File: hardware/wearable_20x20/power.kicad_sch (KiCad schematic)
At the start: 27 parts, among them U1 BQ25185, U2 TPS7A2033PDBVR, U3 TPS63802DLAR, U4 TPS22917DBVR, U5 TPS22917DBVR

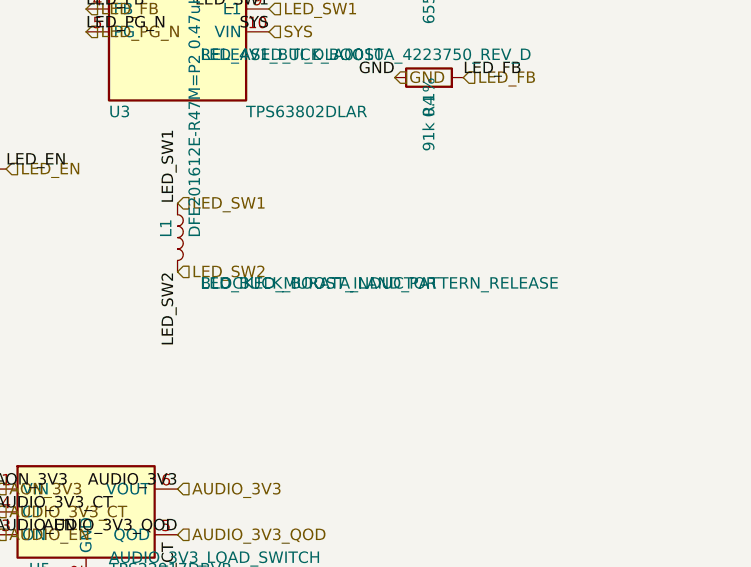
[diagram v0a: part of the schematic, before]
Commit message: Release crystal and power inductor packages
Co-authored-by: illiapliukhin <illiapliukhin@users.noreply.github.com>
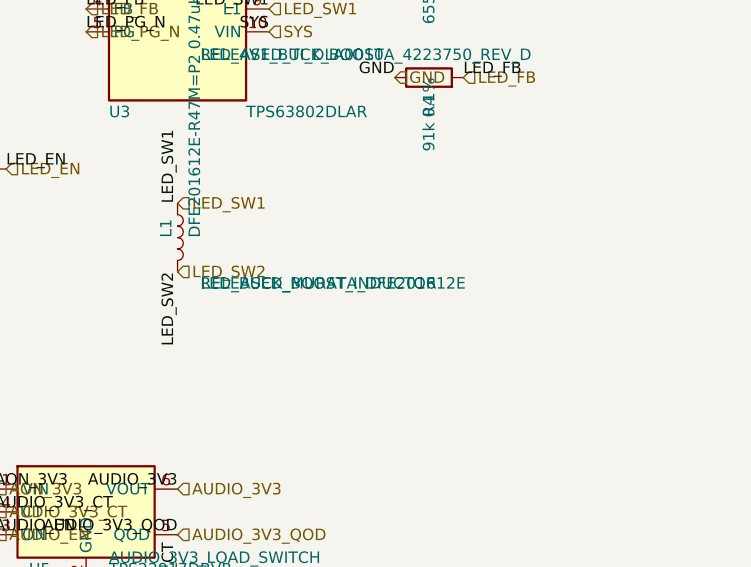
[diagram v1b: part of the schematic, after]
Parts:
- L1: footprint (none) -> PartSignal_Packages:Murata_DFE201612E_2.0x1.6mm; FootprintStatus BLOCKED_MURATA_LAND_PATTERN_RELEASE -> RELEASED_MURATA_DFE201612E
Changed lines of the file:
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@@
 			)
 		)
-		(property "Footprint" ""
+		(property "Footprint" "PartSignal_Packages:Murata_DFE201612E_2.0x1.6mm"
 			(at 157.48 81.28 0)
 			(hide yes)
@@
 			)
 		)
-		(property "FootprintStatus" "BLOCKED_MURATA_LAND_PATTERN_RELEASE"
+		(property "FootprintStatus" "RELEASED_MURATA_DFE201612E"
 			(at 160.02 86.3599 0)
 			(show_name no)
